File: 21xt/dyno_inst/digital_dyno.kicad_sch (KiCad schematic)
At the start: 19 parts, among them J7 Conn_01x04, T1 749013011, U1 MAX14931FASE+, U11 MAX14930FASE+, U2 MAX14930FASE+, U23 CPC1017N

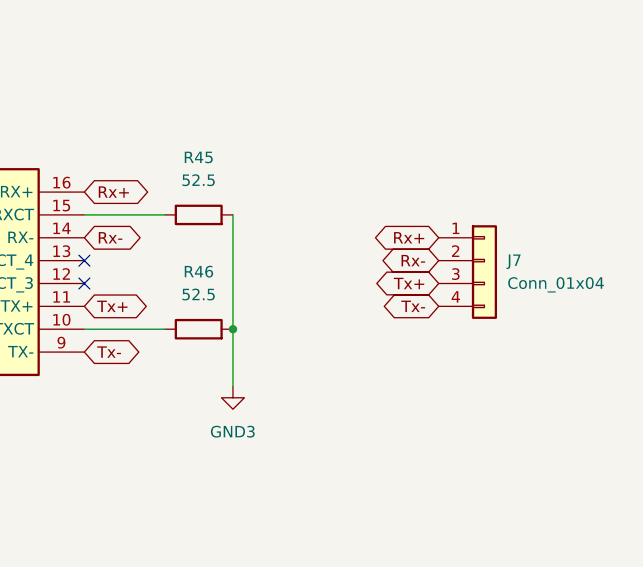
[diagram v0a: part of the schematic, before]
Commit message: dddd
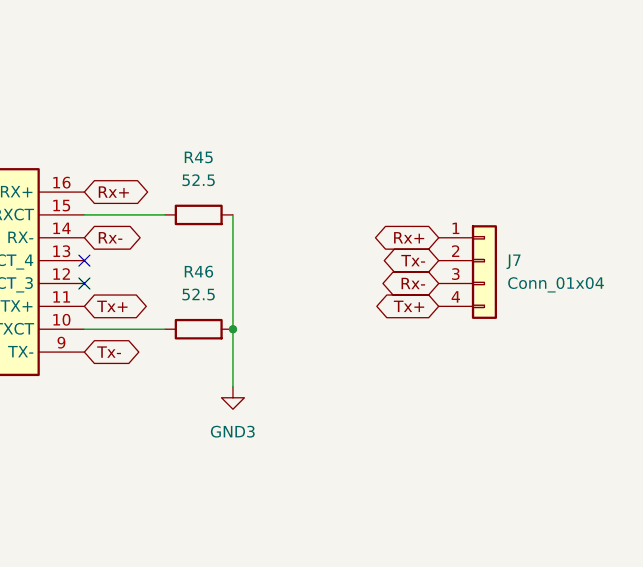
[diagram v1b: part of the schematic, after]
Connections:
- net Rx-: now also J7.3 (Pin_3); no longer J7.2 (Pin_2)
- net Tx+: now also J7.4 (Pin_4); no longer J7.3 (Pin_3)
- net Tx-: now also J7.2 (Pin_2); no longer J7.4 (Pin_4)
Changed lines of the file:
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@@
+		)
+	)
+	(global_label "Rx+"
+		(shape bidirectional)
+		(at 269.24 90.17 180)
+		(fields_autoplaced yes)
+		(effects
+			(font
+				(size 1.27 1.27)
+			)
+			(justify right)
+		)
+		(property "Intersheetrefs" "${INTERSHEET_REFS}"
+			(at 261.273 90.17 0)
+			(effects
+				(font
+					(size 1.27 1.27)
+				)
+				(justify right)
+				(hide yes)
+			)
 		)
 	)
 	(global_label "Tx+"
 		(shape bidirectional)
-		(at 269.24 95.25 180)
-		(fields_autoplaced yes)
-		(effects
-			(font
-				(size 1.27 1.27)
-			)
-			(justify right)
-		)
-		(property "Intersheetrefs" "${INTERSHEET_REFS}"
-			(at 261.5754 95.25 0)
-			(effects
-				(font
-					(size 1.27 1.27)
-				)
-				(justify right)
-				(hide yes)
-			)
-		)
-	)
-	(global_label "Rx+"
-		(shape bidirectional)
-		(at 269.24 90.17 180)
-		(fields_autoplaced yes)
-		(effects
-			(font
-				(size 1.27 1.27)
-			)
-			(justify right)
-		)
-		(property "Intersheetrefs" "${INTERSHEET_REFS}"
-			(at 261.273 90.17 0)
-			(effects
-				(font
-					(size 1.27 1.27)
-				)
-				(justify right)
-				(hide yes)
-			)
-		)
-	)
-	(global_label "Tx+"
-		(shape bidirectional)
 		(at 229.87 97.79 0)
 		(fields_autoplaced yes)
@@
 		)
 	)
+	(global_label "TOPINA3v3"
+		(shape input)
+		(at 45.72 144.78 180)
+		(fields_autoplaced yes)
+		(effects
+			(font
+				(size 1.27 1.27)
+			)
+			(justify right)
+		)
+		(property "Intersheetrefs" "${INTERSHEET_REFS}"
+			(at 32.7562 144.78 0)
+			(effects
+				(font
+					(size 1.27 1.27)
+				)
+				(justify right)
+				(hide yes)
+			)
+		)
+	)
 	(global_label "Tx-"
 		(shape bidirectional)
-		(at 269.24 97.79 180)
-		(fields_autoplaced yes)
-		(effects
-			(font
-				(size 1.27 1.27)
-			)
-			(justify right)
-		)
-		(property "Intersheetrefs" "${INTERSHEET_REFS}"
-			(at 261.5754 97.79 0)
-			(effects
-				(font
-					(size 1.27 1.27)
-				)
-				(justify right)
-				(hide yes)
-			)
-		)
-	)
-	(global_label "TOPINA3v3"
-		(shape input)
-		(at 45.72 144.78 180)
-		(fields_autoplaced yes)
-		(effects
-			(font
-				(size 1.27 1.27)
-			)
-			(justify right)
-		)
-		(property "Intersheetrefs" "${INTERSHEET_REFS}"
-			(at 32.7562 144.78 0)
+		(at 269.24 92.71 180)
+		(fields_autoplaced yes)
+		(effects
+			(font
+				(size 1.27 1.27)
+			)
+			(justify right)
+		)
+		(property "Intersheetrefs" "${INTERSHEET_REFS}"
+			(at 261.5754 92.71 0)
 			(effects
 				(font
@@
 		)
 	)
+	(global_label "Tx+"
+		(shape bidirectional)
+		(at 269.24 97.79 180)
+		(fields_autoplaced yes)
+		(effects
+			(font
+				(size 1.27 1.27)
+			)
+			(justify right)
+		)
+		(property "Intersheetrefs" "${INTERSHEET_REFS}"
+			(at 261.5754 97.79 0)
+			(effects
+				(font
+					(size 1.27 1.27)
+				)
+				(justify right)
+				(hide yes)
+			)
+		)
+	)
 	(global_label "3v3Teensy"
 		(shape input)
@@
 		)
 	)
-	(global_label "Rx-"
-		(shape bidirectional)
-		(at 269.24 92.71 180)
-		(fields_autoplaced yes)
-		(effects
-			(font
-				(size 1.27 1.27)
-			)
-			(justify right)
-		)
-		(property "Intersheetrefs" "${INTERSHEET_REFS}"
-			(at 261.273 92.71 0)
-			(effects
-				(font
-					(size 1.27 1.27)
-				)
-				(justify right)
-				(hide yes)
-			)
-		)
-	)
 	(global_label "Rd+"
 		(shape bidirectional)
@@
 			(effects
 				(font
+					(size 1.27 1.27)
+				)
+				(justify right)
+				(hide yes)
+			)
+		)
+	)
+	(global_label "Rx-"
+		(shape bidirectional)
+		(at 269.24 95.25 180)
+		(fields_autoplaced yes)
+		(effects
+			(font
+				(size 1.27 1.27)
+			)
+			(justify right)
+		)
+		(property "Intersheetrefs" "${INTERSHEET_REFS}"
+			(at 261.273 95.25 0)
+			(effects
+				(font
